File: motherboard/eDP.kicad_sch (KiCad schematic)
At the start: 6 parts, among them J15 20455-040E-76 OLED IPEX, J16 OLED EL POWER, U18 TPS22917DBV

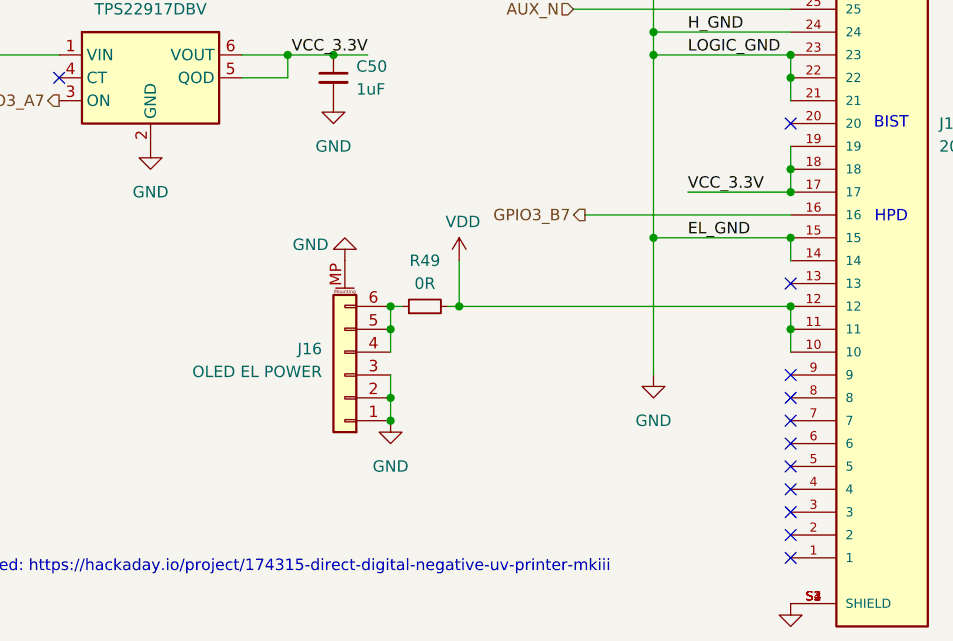
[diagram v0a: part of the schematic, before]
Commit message: v1.0 tapeout and more
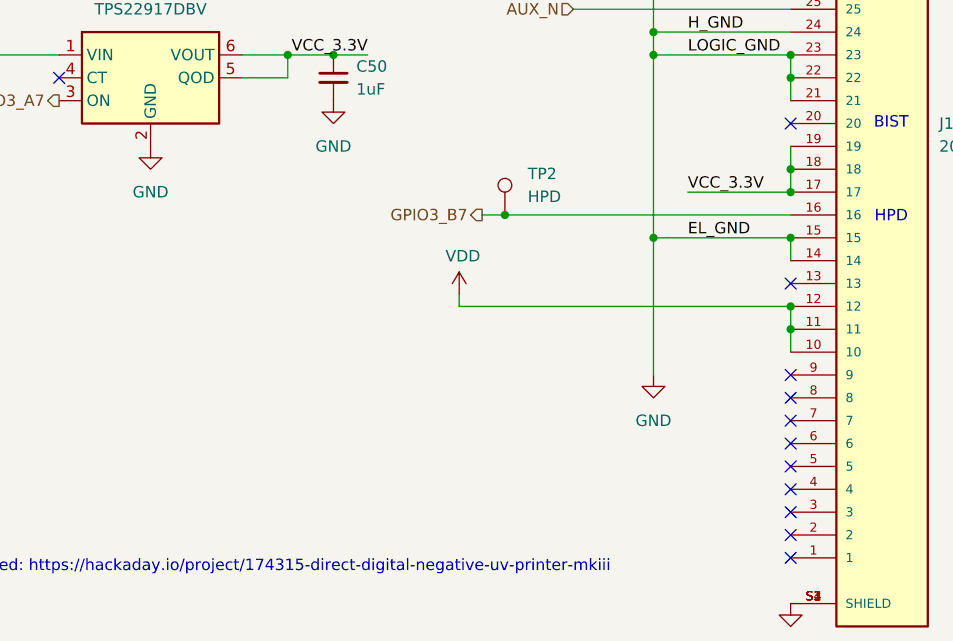
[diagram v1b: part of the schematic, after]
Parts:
- removed J16: OLED EL POWER, 6P_05mm_FPC:FPC-SMD_6P-P0.50_XUNPU_FPC-05F-6PH20, symbol Connector_Generic_MountingPin:Conn_01x06_MountingPin
- removed R49: 0R, Jumper:SolderJumper-2_P1.3mm_Open_TrianglePad1.0x1.5mm, symbol Device:R_Small
- added TP2: HPD, TestPoint:TestPoint_Pad_D1.5mm, symbol Connector:TestPoint
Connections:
- net GPIO3_B7: now also TP2.1
